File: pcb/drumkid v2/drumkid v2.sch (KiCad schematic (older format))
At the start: 43 parts, among them J1 Conn_01x03_Female, J2 Conn_01x03_Female, J3 Conn_01x03_Female, J4 Conn_01x03_Female, J5 Conn_01x05_Female, J6 Conn_01x04_Female, J7 Conn_01x06_Female, J8 Conn_01x05_Female, J9 AudioJack3_Ground_Switch, SW1 SW_SPDT, SW2 SW_Push, SW3 SW_Push, SW4 SW_Push, SW5 SW_Push, SW6 SW_Push, U1 MAX756, U2 ATmega328P-PU, Y1 Crystal

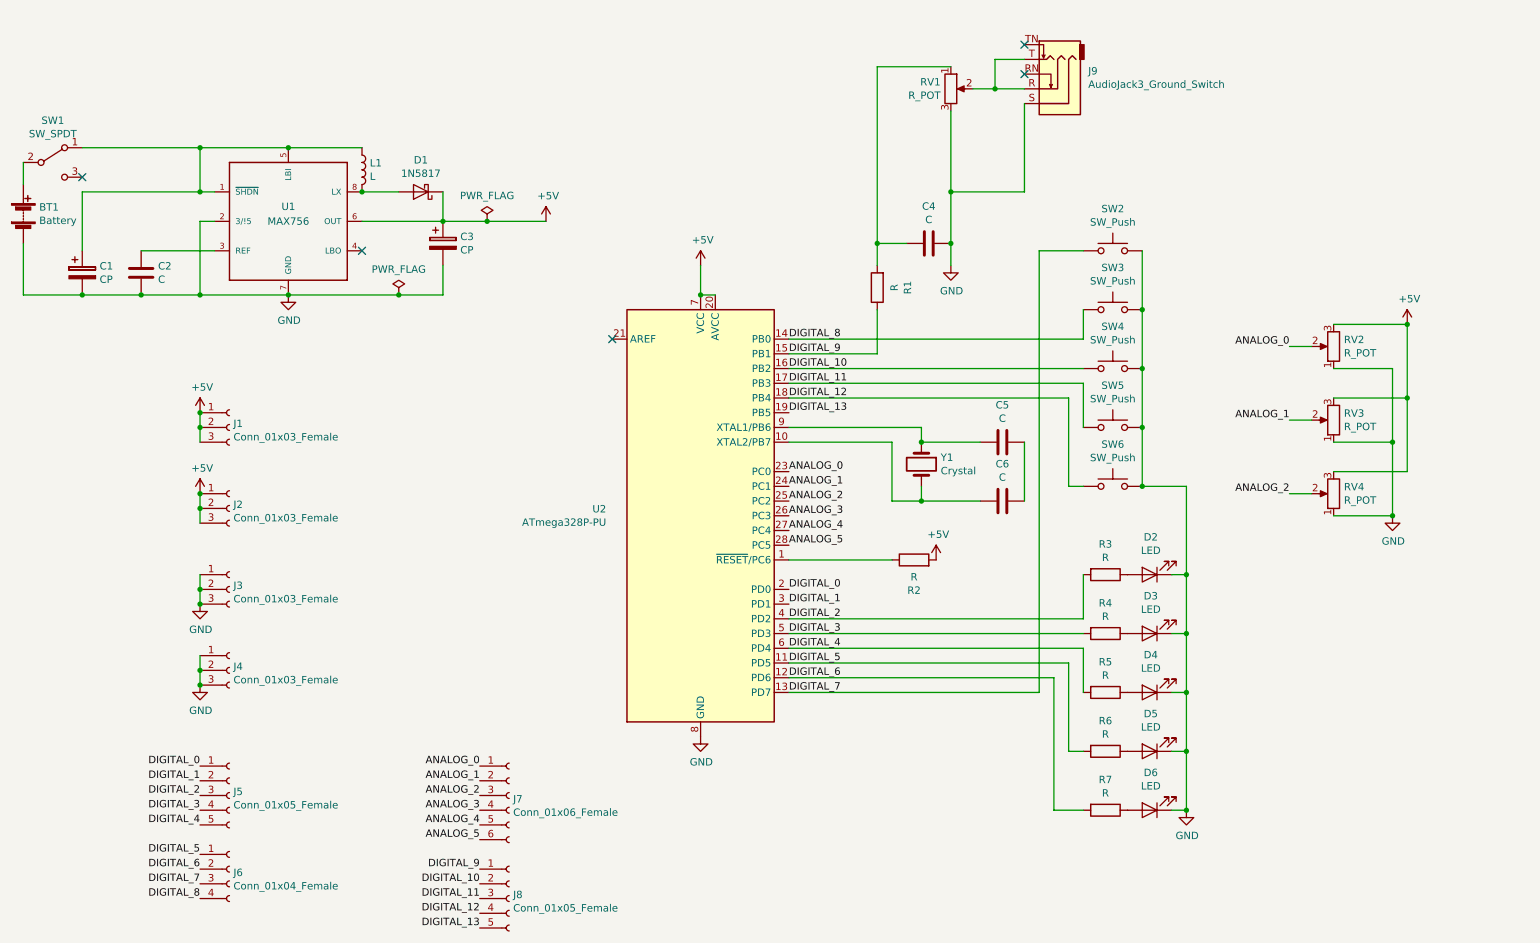
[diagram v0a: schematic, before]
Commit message: more pcb changes, about to do a big-ish change so doing a commit now
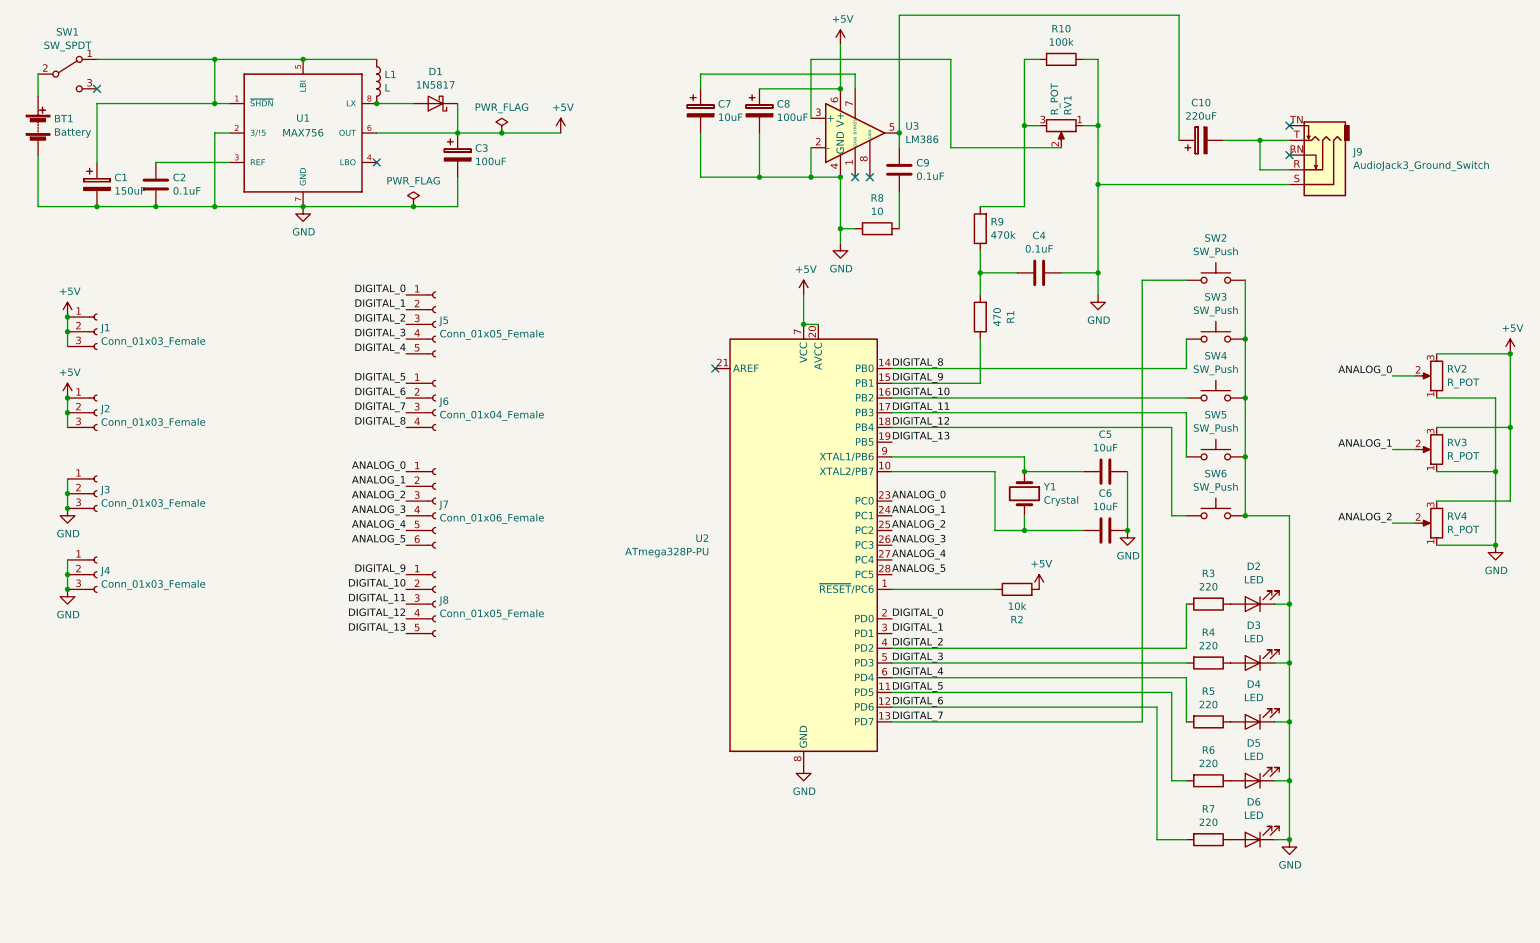
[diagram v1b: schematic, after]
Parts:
- added C10: 220uF, Capacitor_THT:CP_Radial_D6.3mm_P2.50mm, symbol Device:CP
- added C7: 10uF, Capacitor_THT:CP_Radial_D6.3mm_P2.50mm, symbol Device:CP
- added C8: 100uF, Capacitor_THT:CP_Radial_D6.3mm_P2.50mm, symbol Device:CP
- added C9: 0.1uF, Capacitor_THT:C_Disc_D3.4mm_W2.1mm_P2.50mm, symbol Device:C
- added R10: 100k, Resistor_THT:R_Axial_DIN0207_L6.3mm_D2.5mm_P10.16mm_Horizontal, symbol Device:R
- added R8: 10, Resistor_THT:R_Axial_DIN0207_L6.3mm_D2.5mm_P10.16mm_Horizontal, symbol Device:R
- added R9: 470k, Resistor_THT:R_Axial_DIN0207_L6.3mm_D2.5mm_P10.16mm_Horizontal, symbol Device:R
- added U3: LM386, Package_DIP:DIP-8_W7.62mm_Socket, symbol Amplifier_Audio:LM386
- C1: value CP -> 150uF
- C2, C4: value C -> 0.1uF
- C3: value CP -> 100uF
- C5, C6: value C -> 10uF
- R1: value R -> 470
- R2: value R -> 10k
- R3, R4, R5, R6, R7: value R -> 220
- U1: footprint MAX756:SO08 -> Package_DIP:DIP-8_W7.62mm_Socket
- U2: footprint Package_DIP:DIP-28_W7.62mm -> Package_DIP:DIP-28_W7.62mm_Socket
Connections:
- net +5V: now also C8.1, U3.6 (V+)
- net GND: now also C5.2, C6.2, RV1.1, C7.2, C8.2, R10.1, R8.1, U3.2 (-), U3.4 (GND); no longer RV1.3
- net at C4.2, R1.2: now also R9.1; no longer RV1.1
- net at J9.R, J9.T: now also C10.2; no longer RV1.2
- new net: RV1.2, U3.3 (+)
- new net: R10.2, R9.2, RV1.3
- new net: C10.1, C9.1, U3.5
- new net: C7.1, U3.7 (BYPASS)
- new net: C9.2, R8.2
- no-connect marks 5 -> 7
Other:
- moved on the sheet: BT1, C1, C2, C3, C4, C5, C6, D1, D2, D3, D4, D5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
